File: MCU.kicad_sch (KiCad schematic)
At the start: 46 parts, among them SW1 SW_Push, U1 STM32F429IGTx, Y1 32.768KHz, Y2 25MHz

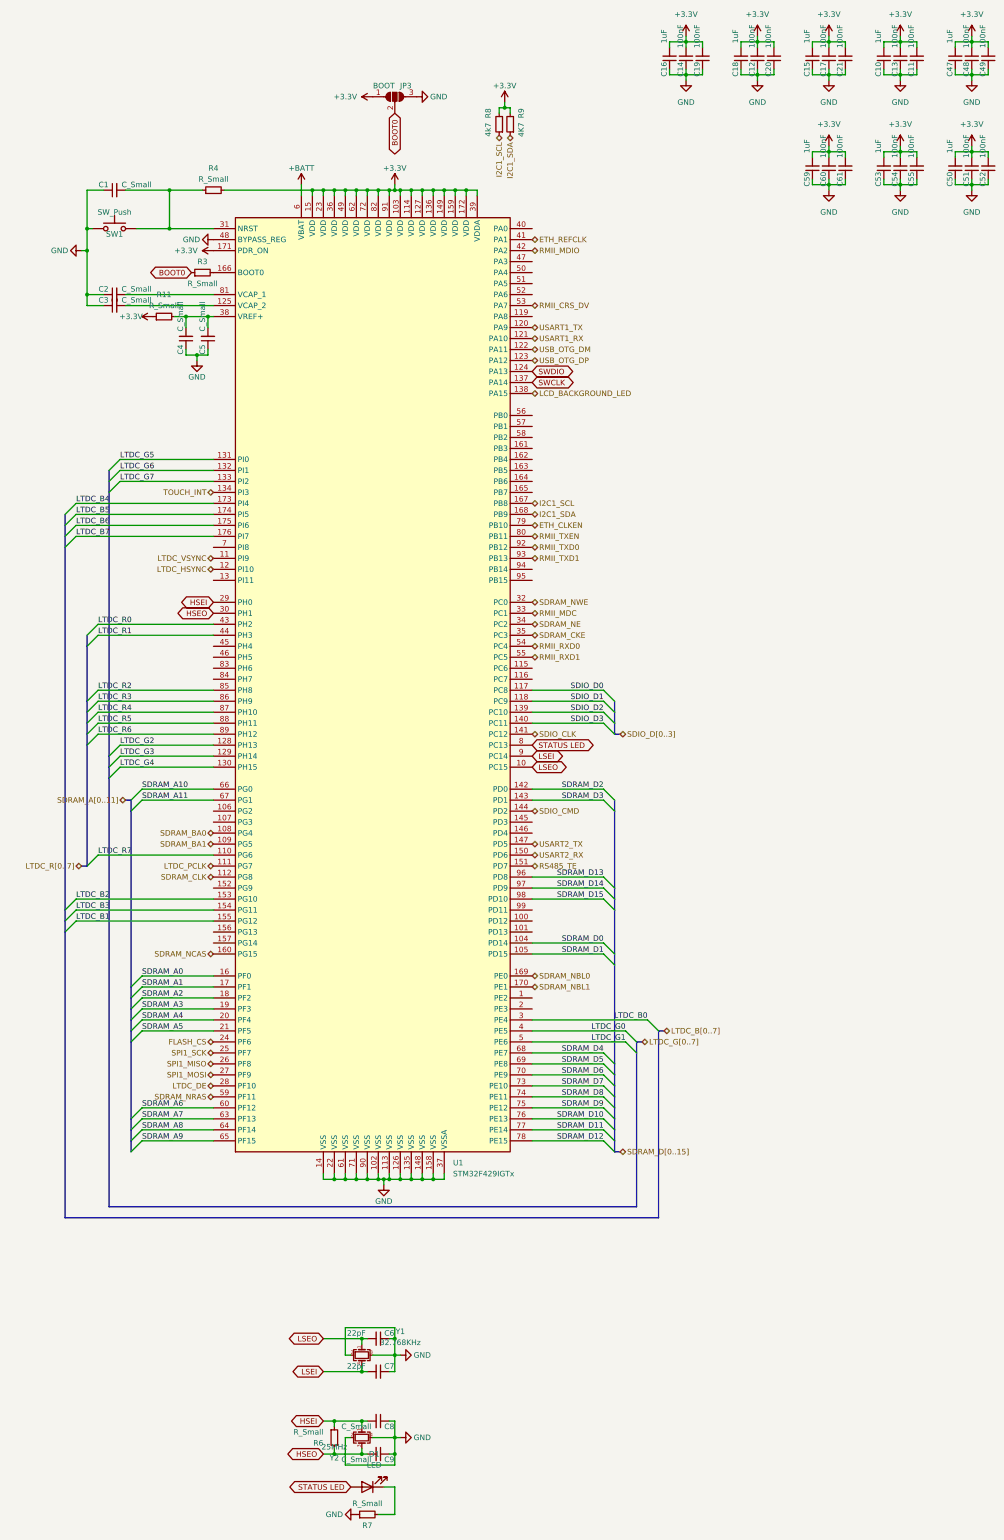
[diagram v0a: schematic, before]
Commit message: Finish USB, LoRa Layout
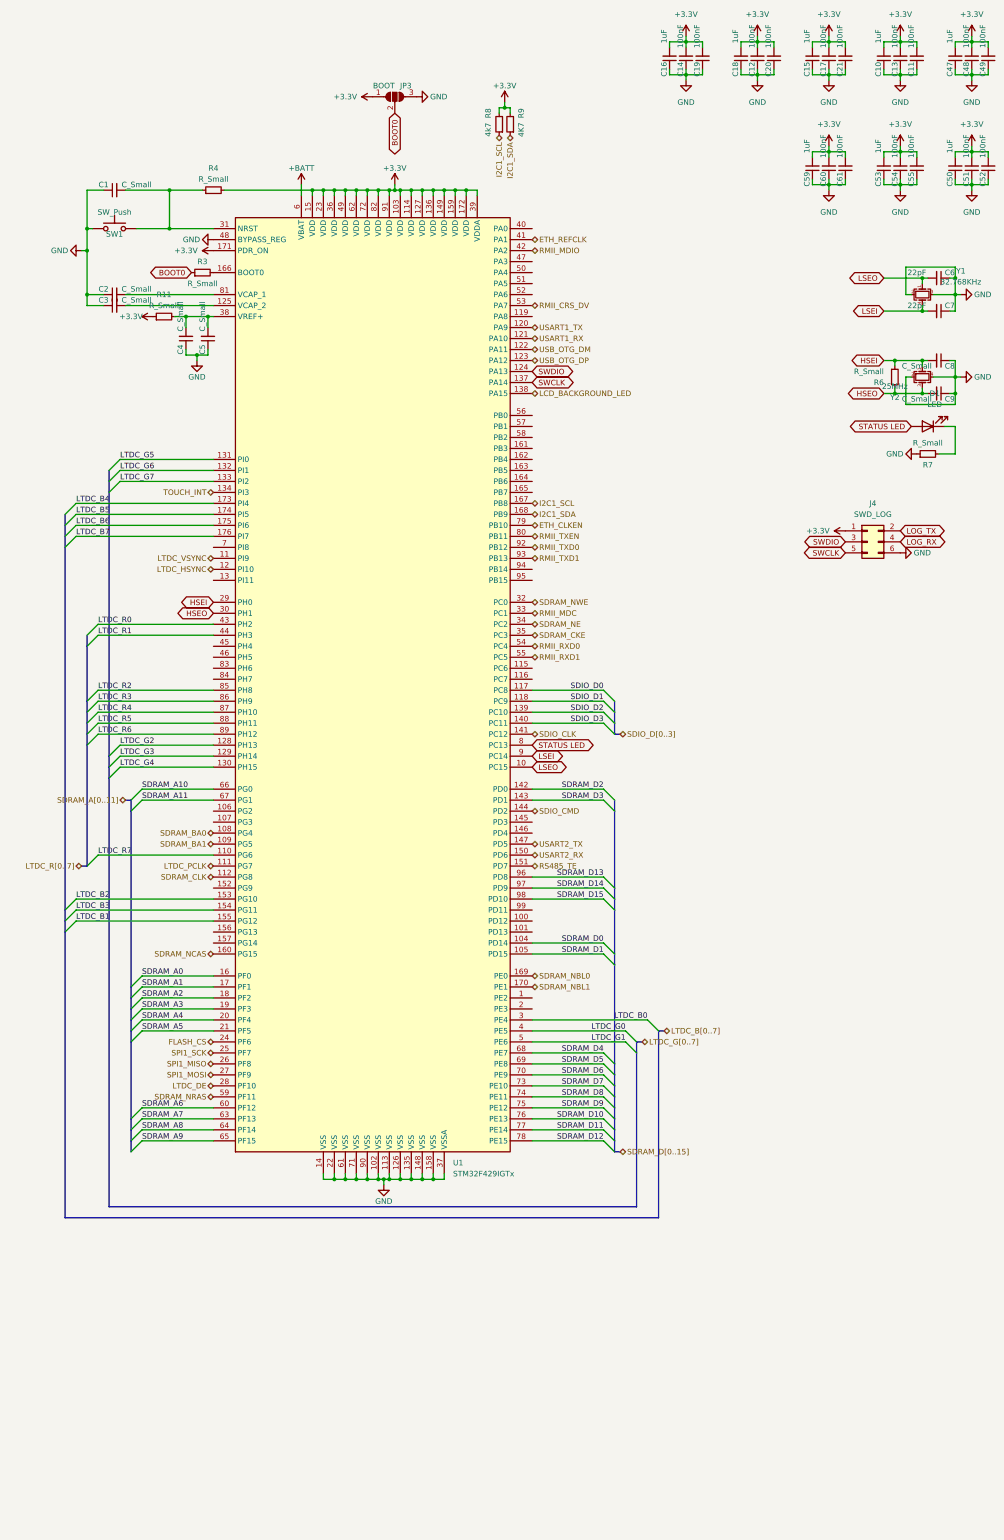
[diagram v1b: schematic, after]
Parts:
- added J4: SWD_LOG, Connector_PinHeader_2.54mm:PinHeader_2x03_P2.54mm_Horizontal, symbol Connector_Generic:Conn_02x03_Odd_Even
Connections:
- net +3.3V: now also J4.1 (Pin_1)
- net GND: now also J4.6 (Pin_6)
- net SWCLK: now also J4.5 (Pin_5)
- net SWDIO: now also J4.3 (Pin_3)
- new net LOG_RX: J4.4 (Pin_4)
- new net LOG_TX: J4.2 (Pin_2)
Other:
- moved on the sheet: C6, C7, C8, C9, D1, R6, R7, Y1, Y2
